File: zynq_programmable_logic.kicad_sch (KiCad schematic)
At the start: 0 parts

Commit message: sch updated zynq ddr
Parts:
- added D500: RED, LED_0402_RED, symbol Schematic-Lib-PhilsLab:LED_0402_RED
- added Q500: T2N7002AK, Package_TO_SOT_SMD:SOT-23, symbol Transistor_FET:T2N7002AK
- added R500: 1k, Resistor_SMD:R_0402_1005Metric, symbol Device:R
- added R501: 100k, Resistor_SMD:R_0402_1005Metric, symbol Device:R
- added R502: 12K, Resistor_SMD:R_0402_1005Metric, symbol Device:R
- added R503: 510, Resistor_SMD:R_0402_1005Metric, symbol Device:R
- added U1: XC7Z020-2CLG400I, Package_BGA:Xilinx_CLG400, symbol 2024-11-30_12-42-37:XC7Z020-2CLG400I
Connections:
- new net +3V3: R500.1, R503.2
- new net FET_PL_G: Q500.1 (G), R502.1
- new net GND: Q500.2 (S), R501.2
- new net LED_PL: R501.1, R502.2, U1.T12 (IO_L2P_T0_34)
- new net LED_PL_K: D500.A, D500.K, Q500.3 (D), R503.1
- new net NPUDC: R500.2, U1.U13 (IO_L3P_T0_DQS_PUDC_B_34)
- new net PL_B34_L10_N: U1.W15 (IO_L10N_T1_34)
- new net PL_B34_L10_P: U1.V15 (IO_L10P_T1_34)
- new net PL_B34_L11_N: U1.P20 (IO_L14N_T2_SRCC_34), U1.U15 (IO_L11N_T1_SRCC_34)
- new net PL_B34_L11_P: U1.U14 (IO_L11P_T1_SRCC_34)
- new net PL_B34_L14_P: U1.N20 (IO_L14P_T2_SRCC_34)
- new net PL_B34_L15_N: U1.U20 (IO_L15N_T2_DQS_34)
- new net PL_B34_L15_P: U1.T20 (IO_L15P_T2_DQS_34)
- new net PL_B34_L16_N: U1.W20 (IO_L16N_T2_34)
- new net PL_B34_L16_P: U1.V20 (IO_L16P_T2_34)
- new net PL_B34_L17_N: U1.Y19 (IO_L17N_T2_34)
- new net PL_B34_L17_P: U1.Y18 (IO_L17P_T2_34)
- new net PL_B34_L18_N: U1.W16 (IO_L18N_T2_34)
- new net PL_B34_L18_P: U1.V16 (IO_L18P_T2_34)
- new net PL_B34_L4_N: U1.W13 (IO_L4N_T0_34)
- new net PL_B34_L4_P: U1.V12 (IO_L4P_T0_34)
- new net PL_B34_L7_N: U1.Y17 (IO_L7N_T1_34)
- new net PL_B34_L7_P: U1.Y16 (IO_L7P_T1_34)
- new net PL_B34_L8_N: U1.Y14 (IO_L8N_T1_34)
- new net PL_B34_L8_P: U1.W14 (IO_L8P_T1_34)
- new net PL_B35_L11_P: U1.L17 (IO_L11N_T1_SRCC_35)
- new net PL_B35_L13_N: U1.H17 (IO_L13N_T2_MRCC_35)
- new net PL_B35_L13_P: U1.H16 (IO_L13P_T2_MRCC_35)
- new net PL_B35_L14_N: U1.H18 (IO_L14N_T2_AD4N_SRCC_35)
- new net PL_B35_L14_P: U1.J18 (IO_L14P_T2_AD4P_SRCC_35)
- new net PL_B35_L16_N: U1.G18 (IO_L16N_T2_35)
- new net PL_B35_L16_P: U1.G17 (IO_L16P_T2_35)
- new net PL_B35_L20_N: U1.J14 (IO_L20N_T3_AD6N_35)
- new net PL_B35_L20_P: U1.K14 (IO_L20P_T3_AD6P_35)
- new net PL_B35_L22_N: U1.L15 (IO_L22N_T3_AD7N_35)
- new net PL_B35_L22_P: U1.L14 (IO_L22P_T3_AD7P_35)
- new net PL_B35_L24_N: U1.J16 (IO_L24N_T3_AD15N_35)
- new net PL_B35_L3_N: U1.D18 (IO_L3N_T0_DQS_AD1N_35)
- new net PL_B35_L3_P: U1.E17 (IO_L3P_T0_DQS_AD1P_35)
- new net PL_B35_L5_N: U1.E19 (IO_L5N_T0_AD9N_35)
- new net PL_B35_L5_P: U1.E18 (IO_L5P_T0_AD9P_35)
- new net PL_B35_L6_P: U1.F16 (IO_L6P_T0_35)
- new net PL_B35_L7_N: U1.M20 (IO_L7N_T1_AD2N_35)
- new net PL_B35_L7_P: U1.M19 (IO_L7P_T1_AD2P_35)
- new net PL_B35_L8_N: U1.M18 (IO_L8N_T1_AD10N_35)
- new net PL_B35_L8_P: U1.M17 (IO_L8P_T1_AD10P_35)
- new net PL_B35_L9_N: U1.L20 (IO_L9N_T1_DQS_AD3N_35)
- new net PL_B35_L9_P: U1.L19 (IO_L9P_T1_DQS_AD3P_35)
- new net PL_CLK_125MHZ: U1.K17 (IO_L12P_T1_MRCC_35)
- no-connect marks 0 -> 16

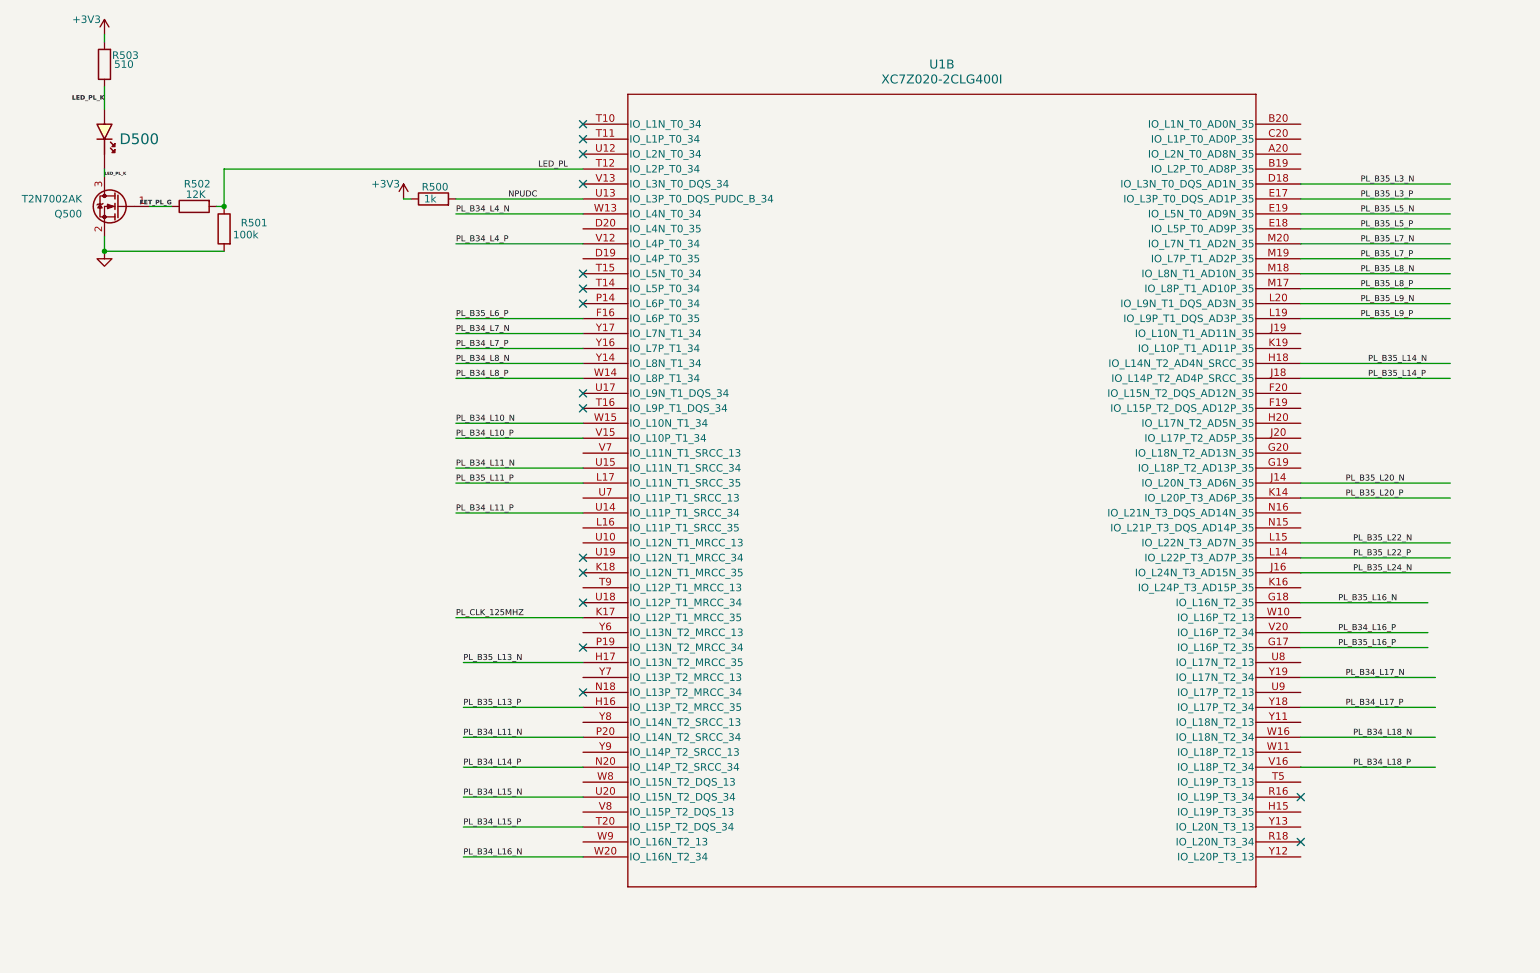
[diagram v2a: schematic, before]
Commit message: all page
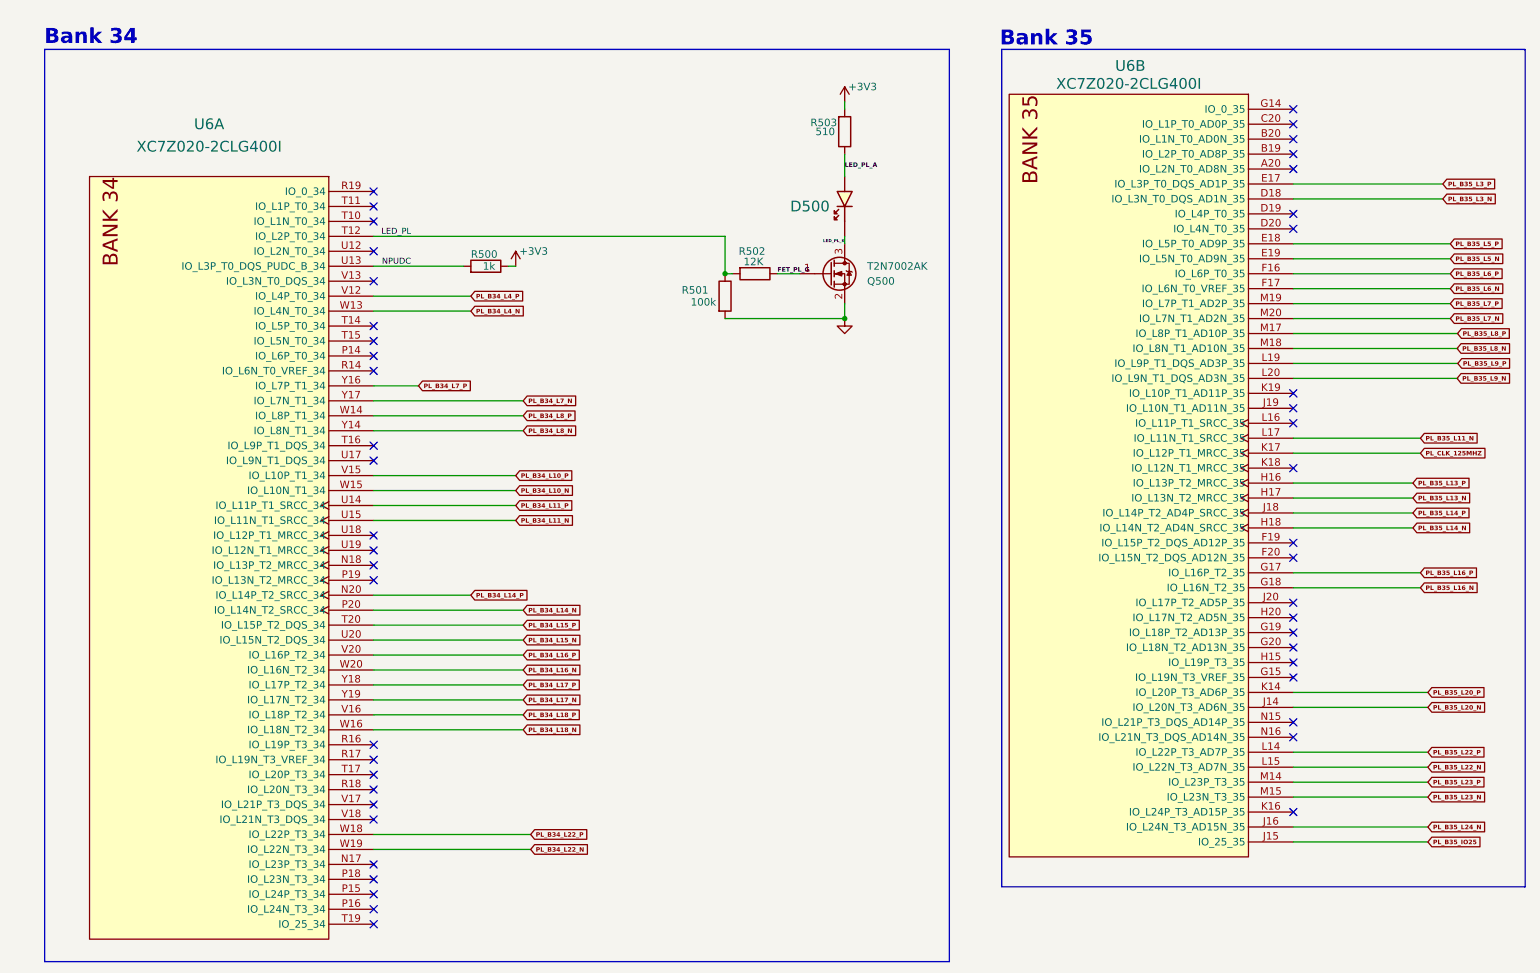
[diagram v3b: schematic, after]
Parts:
- removed U1: XC7Z020-2CLG400I, Package_BGA:Xilinx_CLG400, symbol 2024-11-30_12-42-37:XC7Z020-2CLG400I
- added U6: XC7Z020-2CLG400I, zynq_sc7z0x0:CLG400, symbol Zynq_xc7z0x0-x:CMP-0363-00007-3
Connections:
- net LED_PL: now also U6.T12 (IO_L2P_T0_34)
- net LED_PL_K: no longer D500.A, R503.1
- net NPUDC: now also U6.U13 (IO_L3P_T0_DQS_PUDC_B_34)
- net PL_B34_L10_N: now also U6.W15 (IO_L10N_T1_34)
- net PL_B34_L10_P: now also U6.V15 (IO_L10P_T1_34)
- net PL_B34_L11_N: now also U6.U15 (IO_L11N_T1_SRCC_34)
- net PL_B34_L11_P: now also U6.U14 (IO_L11P_T1_SRCC_34)
- net PL_B34_L14_P: now also U6.N20 (IO_L14P_T2_SRCC_34)
- net PL_B34_L15_N: now also U6.U20 (IO_L15N_T2_DQS_34)
- net PL_B34_L15_P: now also U6.T20 (IO_L15P_T2_DQS_34)
- net PL_B34_L16_N: now also U6.W20 (IO_L16N_T2_34)
- net PL_B34_L16_P: now also U6.V20 (IO_L16P_T2_34)
- net PL_B34_L17_N: now also U6.Y19 (IO_L17N_T2_34)
- net PL_B34_L17_P: now also U6.Y18 (IO_L17P_T2_34)
- net PL_B34_L18_N: now also U6.W16 (IO_L18N_T2_34)
- net PL_B34_L18_P: now also U6.V16 (IO_L18P_T2_34)
- net PL_B34_L4_N: now also U6.W13 (IO_L4N_T0_34)
- net PL_B34_L4_P: now also U6.V12 (IO_L4P_T0_34)
- net PL_B34_L7_N: now also U6.Y17 (IO_L7N_T1_34)
- net PL_B34_L7_P: now also U6.Y16 (IO_L7P_T1_34)
- net PL_B34_L8_N: now also U6.Y14 (IO_L8N_T1_34)
- net PL_B34_L8_P: now also U6.W14 (IO_L8P_T1_34)
- net PL_B35_L13_N: now also U6.H17 (IO_L13N_T2_MRCC_35)
- net PL_B35_L13_P: now also U6.H16 (IO_L13P_T2_MRCC_35)
- net PL_B35_L14_N: now also U6.H18 (IO_L14N_T2_AD4N_SRCC_35)
- net PL_B35_L14_P: now also U6.J18 (IO_L14P_T2_AD4P_SRCC_35)
- net PL_B35_L16_N: now also U6.G18 (IO_L16N_T2_35)
- net PL_B35_L16_P: now also U6.G17 (IO_L16P_T2_35)
- net PL_B35_L20_N: now also U6.J14 (IO_L20N_T3_AD6N_35)
- net PL_B35_L20_P: now also U6.K14 (IO_L20P_T3_AD6P_35)
- net PL_B35_L22_N: now also U6.L15 (IO_L22N_T3_AD7N_35)
- net PL_B35_L22_P: now also U6.L14 (IO_L22P_T3_AD7P_35)
- net PL_B35_L24_N: now also U6.J16 (IO_L24N_T3_AD15N_35)
- net PL_B35_L3_N: now also U6.D18 (IO_L3N_T0_DQS_AD1N_35)
- net PL_B35_L3_P: now also U6.E17 (IO_L3P_T0_DQS_AD1P_35)
- net PL_B35_L5_N: now also U6.E19 (IO_L5N_T0_AD9N_35)
- net PL_B35_L5_P: now also U6.E18 (IO_L5P_T0_AD9P_35)
- net PL_B35_L6_P: now also U6.F16 (IO_L6P_T0_35)
- net PL_B35_L7_N: now also U6.M20 (IO_L7N_T1_AD2N_35)
- net PL_B35_L7_P: now also U6.M19 (IO_L7P_T1_AD2P_35)
- net PL_B35_L8_N: now also U6.M18 (IO_L8N_T1_AD10N_35)
- net PL_B35_L8_P: now also U6.M17 (IO_L8P_T1_AD10P_35)
- net PL_B35_L9_N: now also U6.L20 (IO_L9N_T1_DQS_AD3N_35)
- net PL_B35_L9_P: now also U6.L19 (IO_L9P_T1_DQS_AD3P_35)
- net PL_CLK_125MHZ: now also U6.K17 (IO_L12P_T1_MRCC_35)
- new net LED_PL_A: D500.A, R503.1
- new net PL_B34_L14_N: U6.P20 (IO_L14N_T2_SRCC_34)
- new net PL_B34_L22_N: U6.W19 (IO_L22N_T3_34)
- new net PL_B34_L22_P: U6.W18 (IO_L22P_T3_34)
- new net PL_B35_IO25: U6.J15 (IO_25_35)
- new net PL_B35_L11_N: U6.L17 (IO_L11N_T1_SRCC_35)
- new net PL_B35_L23_N: U6.M15 (IO_L23N_T3_35)
- new net PL_B35_L23_P: U6.M14 (IO_L23P_T3_35)
- new net PL_B35_L6_N: U6.F17 (IO_L6N_T0_VREF_35)
- no-connect marks 16 -> 48
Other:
- note added: "Bank 34"
- note added: "Bank 35"
- title: (none) -> Zynq Programmable Logic (PL)
- moved on the sheet: D500, Q500, R500, R501, R502, R503

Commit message: sch-to-pcb
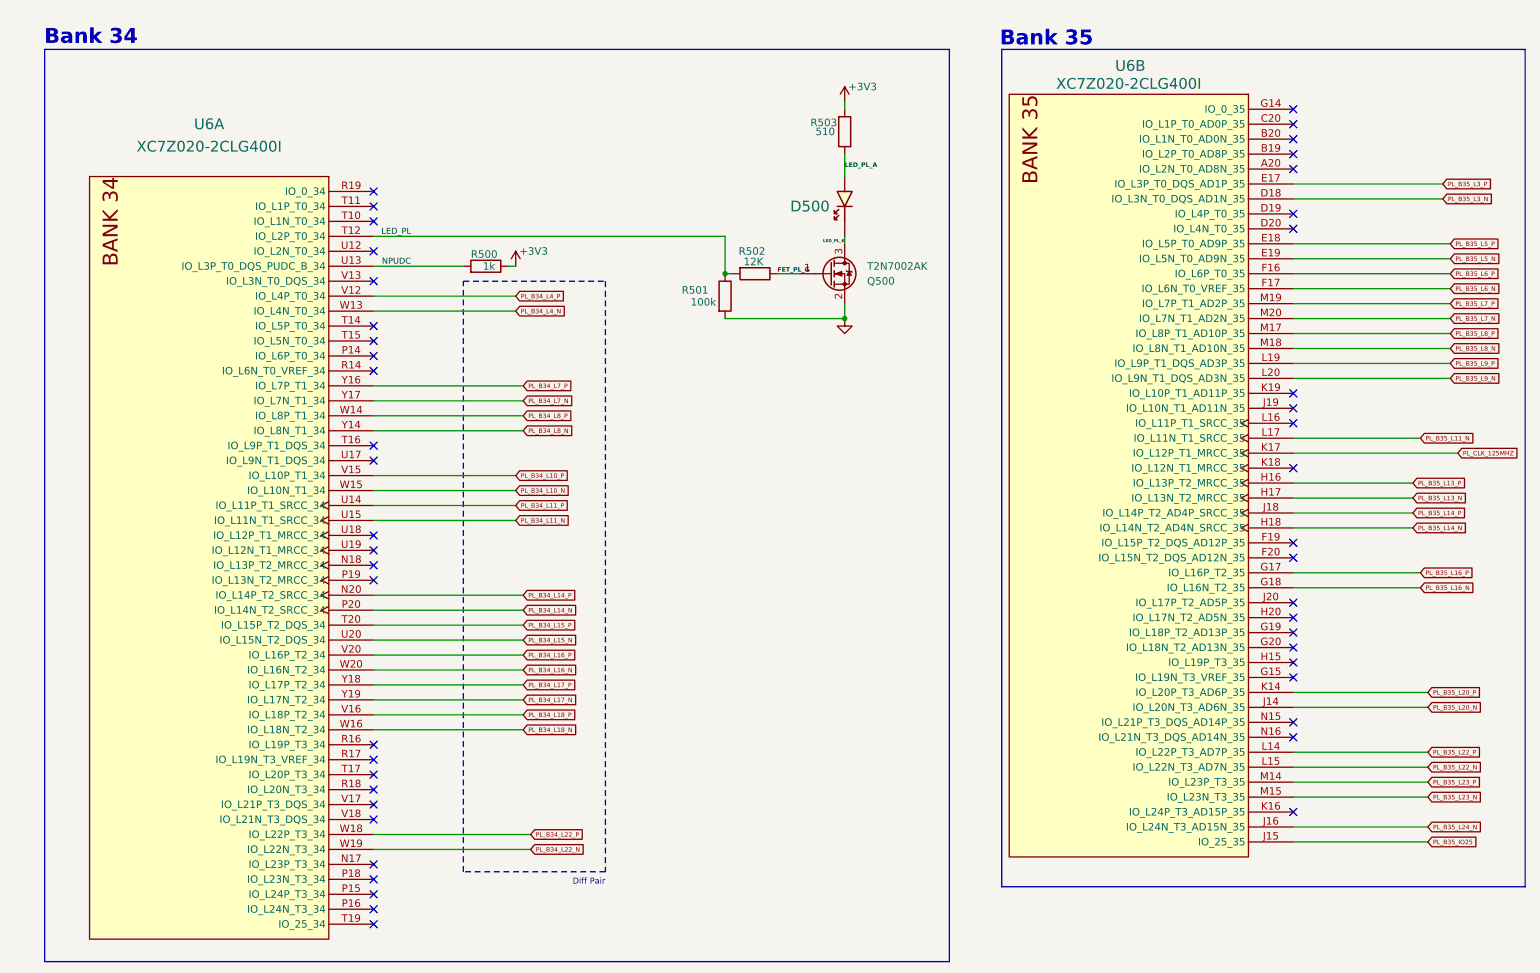
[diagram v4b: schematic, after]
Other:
- note added: "Diff Pair"

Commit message: xc7z020-fanout
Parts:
- U6: footprint zynq_sc7z0x0:CLG400 -> Package_BGA:Xilinx_CLG400
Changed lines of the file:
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@@
 			)
 		)
-		(property "Footprint" "zynq_sc7z0x0:CLG400"
+		(property "Footprint" "Package_BGA:Xilinx_CLG400"
 			(at 26.67 41.91 0)
 			(effects
@@
 			)
 		)
-		(property "Footprint" "zynq_sc7z0x0:CLG400"
+		(property "Footprint" "Package_BGA:Xilinx_CLG400"
 			(at 182.88 27.94 0)
 			(effects

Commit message: ram-update
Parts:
- D500: footprint LED_0402_RED -> Footprint-Lib-PhilsLab:LED_0402_RED
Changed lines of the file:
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@@
 			)
 		)
-		(property "Footprint" "LED_0402_RED"
+		(property "Footprint" "Footprint-Lib-PhilsLab:LED_0402_RED"
 			(at 154.94 46.99 0)
 			(effects
